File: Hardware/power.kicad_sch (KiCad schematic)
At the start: 15 parts, among them U4 TPS54308, U5 AMS1117-3.3

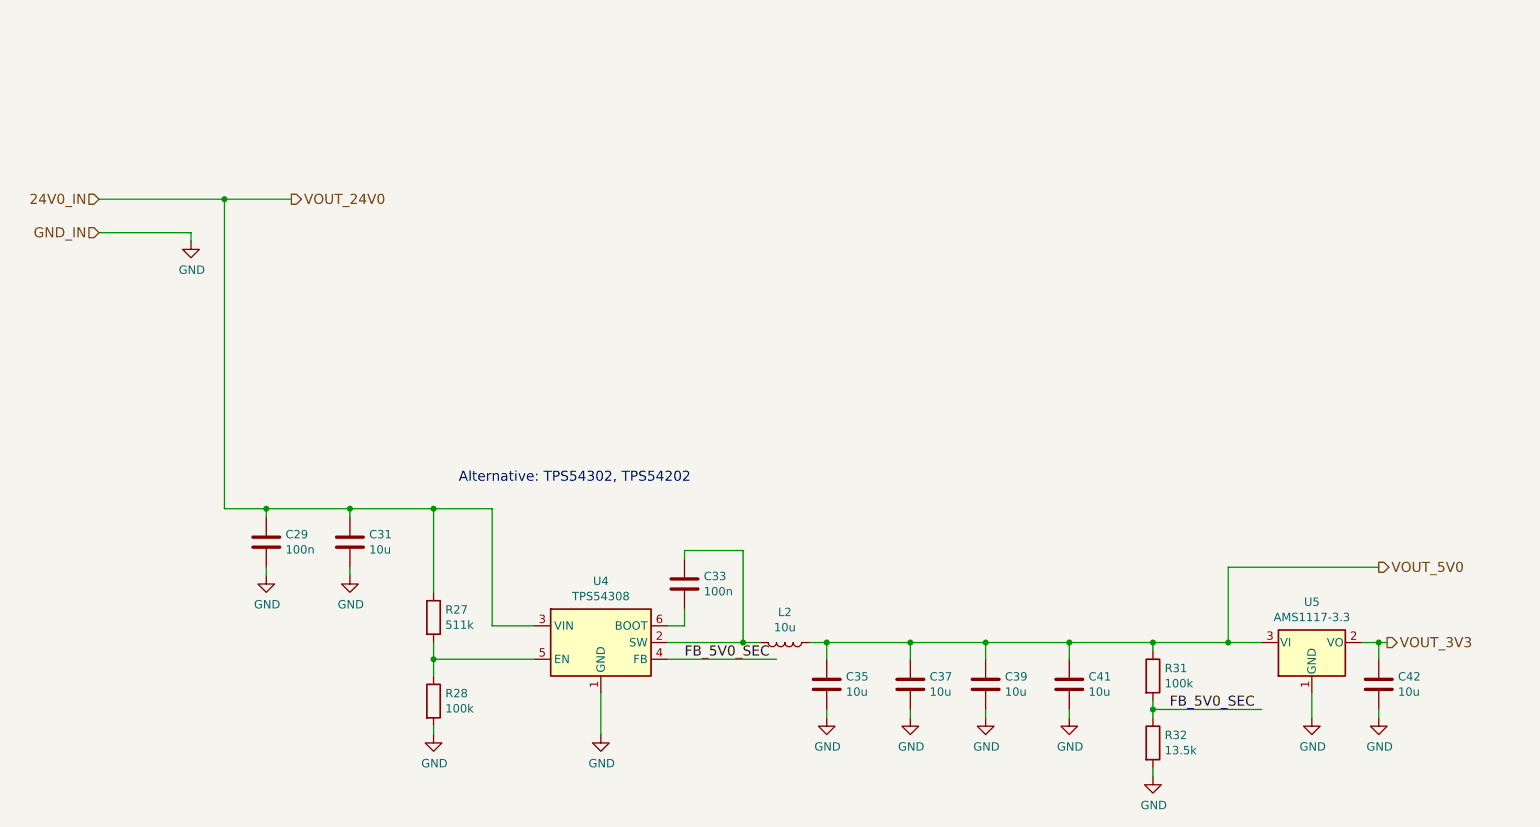
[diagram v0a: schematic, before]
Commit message: Updated power supply
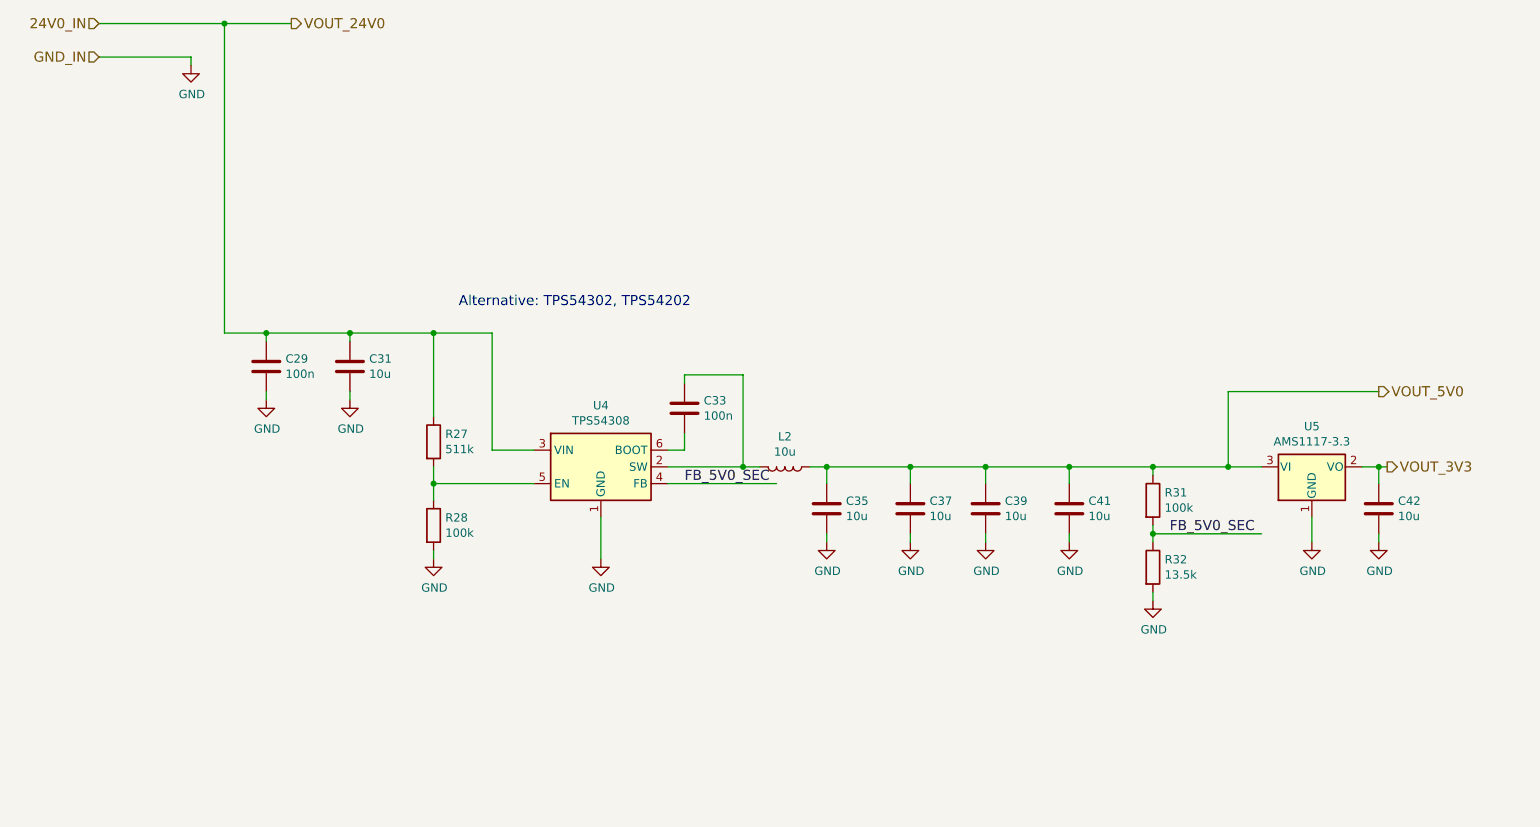
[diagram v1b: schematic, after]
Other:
- moved on the sheet: C29, C31, C33, C35, C37, C39, C41, C42, L2, R27, R28, R31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

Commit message: chore: cleanup
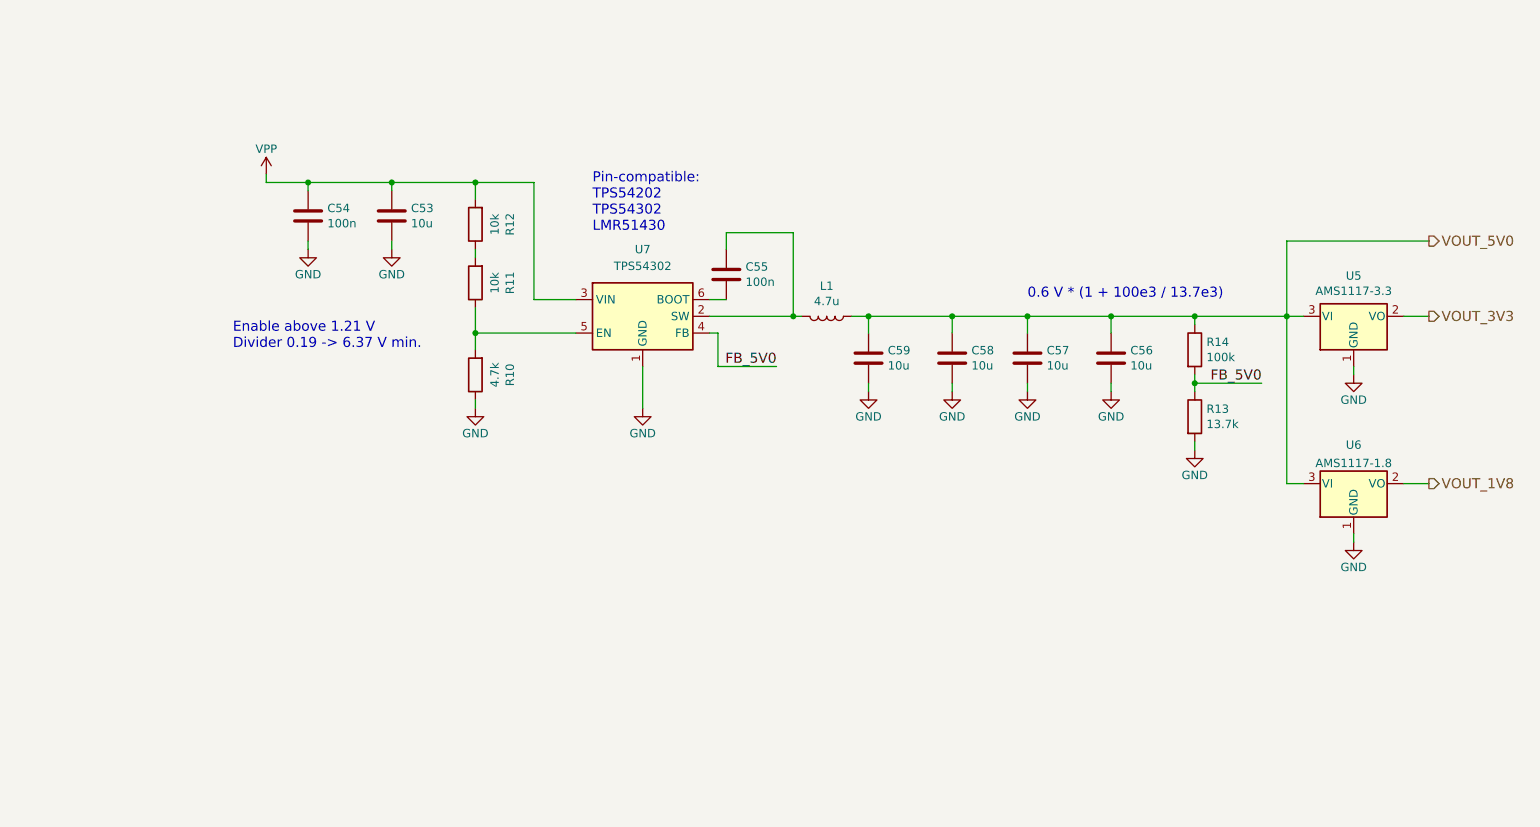
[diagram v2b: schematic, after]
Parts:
- removed C29, C33: 100n, Capacitor_SMD:C_0603_1608Metric_Pad1.08x0.95mm_HandSolder, symbol Device:C
- removed C31, C35, C37, C39, C41, C42: 10u, Capacitor_SMD:C_1206_3216Metric_Pad1.33x1.80mm_HandSolder, symbol Device:C
- removed L2: 10u, Inductor_SMD:L_Abracon_ASPI-0630LR, symbol Device:L
- removed R27: 511k, Resistor_SMD:R_0603_1608Metric_Pad0.98x0.95mm_HandSolder, symbol Device:R
- removed R28, R31: 100k, Resistor_SMD:R_0603_1608Metric_Pad0.98x0.95mm_HandSolder, symbol Device:R
- removed R32: 13.5k, Resistor_SMD:R_0603_1608Metric_Pad0.98x0.95mm_HandSolder, symbol Device:R
- removed U4: TPS54308, Package_TO_SOT_SMD:SOT-23-6, symbol Regulator_Switching:TPS54308
- added C53, C56, C57, C58, C59: 10u, Capacitor_SMD:C_1206_3216Metric, symbol Device:C
- added C54, C55: 100n, Capacitor_SMD:C_0402_1005Metric, symbol Device:C
- added L1: 4.7u, Inductor_SMD:L_Abracon_ASPI-0630LR, symbol Device:L
- added R10: 4.7k, Resistor_SMD:R_0402_1005Metric, symbol Device:R
- added R11, R12: 10k, Resistor_SMD:R_0402_1005Metric, symbol Device:R
- added R13: 13.7k, Resistor_SMD:R_0402_1005Metric, symbol Device:R
- added R14: 100k, Resistor_SMD:R_0402_1005Metric, symbol Device:R
- added U6: AMS1117-1.8, Package_TO_SOT_SMD:SOT-223-3_TabPin2, symbol Regulator_Linear:AMS1117-1.8
- added U7: TPS54302, Package_TO_SOT_SMD:SOT-23-6, symbol Regulator_Switching:TPS54302
- U5: JLCPCB Rotation Offset (none) -> 180; MPN (none) -> C6186
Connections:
- net GND: now also C53.2, C54.2, C56.2, C57.2, C58.2, C59.2, R10.1, R13.2, U6.1 (GND), U7.1 (GND)
- net VOUT_5V0: now also C56.1, C57.1, C58.1, C59.1, L1.1, R14.1, U6.3 (VI)
- new net: C55.1, L1.2, U7.2 (SW)
- new net: C55.2, U7.6 (BOOT)
- new net: R10.2, R11.1, U7.5 (EN)
- new net: R11.2, R12.1
- new net FB_5V0: R13.1, R14.2, U7.4 (FB)
- new net VOUT_1V8: U6.2 (VO)
- new net VPP: C53.1, C54.1, R12.2, U7.3 (VIN)
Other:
- note added: "0.6 V * (1 + 100e3 / 13.7e3)"
- note added: "Enable above 1.21 V Divider 0.19 -> 6.37 V min."
- note added: "Pin-compatible: TPS54202 TPS54302 LMR51430"
- note removed: "Alternative: TPS54302, TPS54202"
- title: Supply -> (none)
